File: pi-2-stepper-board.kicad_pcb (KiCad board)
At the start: 2 copper layers, 65 x 56 mm, 21 parts, among them CON1 DC12v, P1 Servo (A0), P2 Endstop1 (A1), P3 Endstop2 (A2), P4 Stepper1, P5 Stepper2, P6 COM, P7 Aux1 (D10 - 13), P8 Aux2 (I2C), SW1 SW_PUSH, SW2 SPDT, U1 Pi2_3_GPIO, U2 Arduino_Pro_Mini_3v3_8MHz, U3 STEPSTICK, U4 STEPSTICK, U5 DC2DC

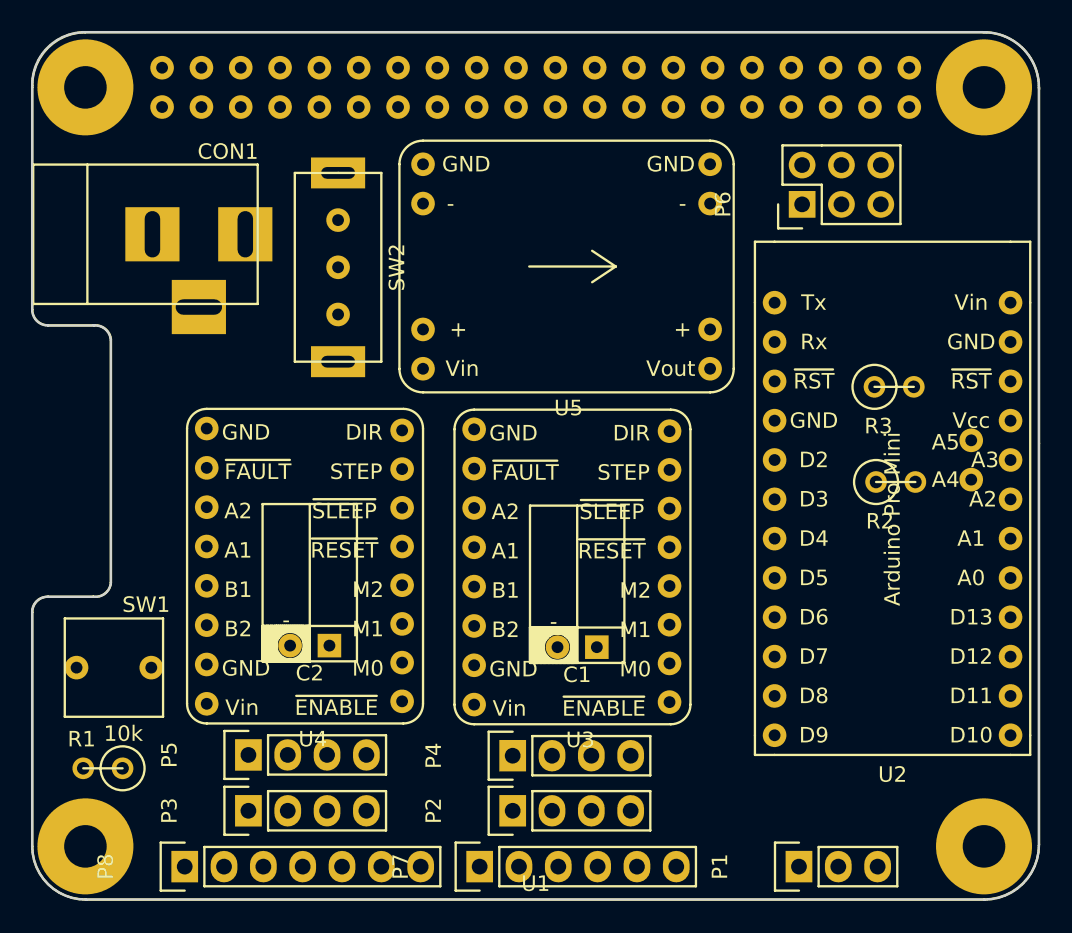
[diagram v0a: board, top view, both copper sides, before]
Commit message: Clean up repo - board 1.0a non hat spec
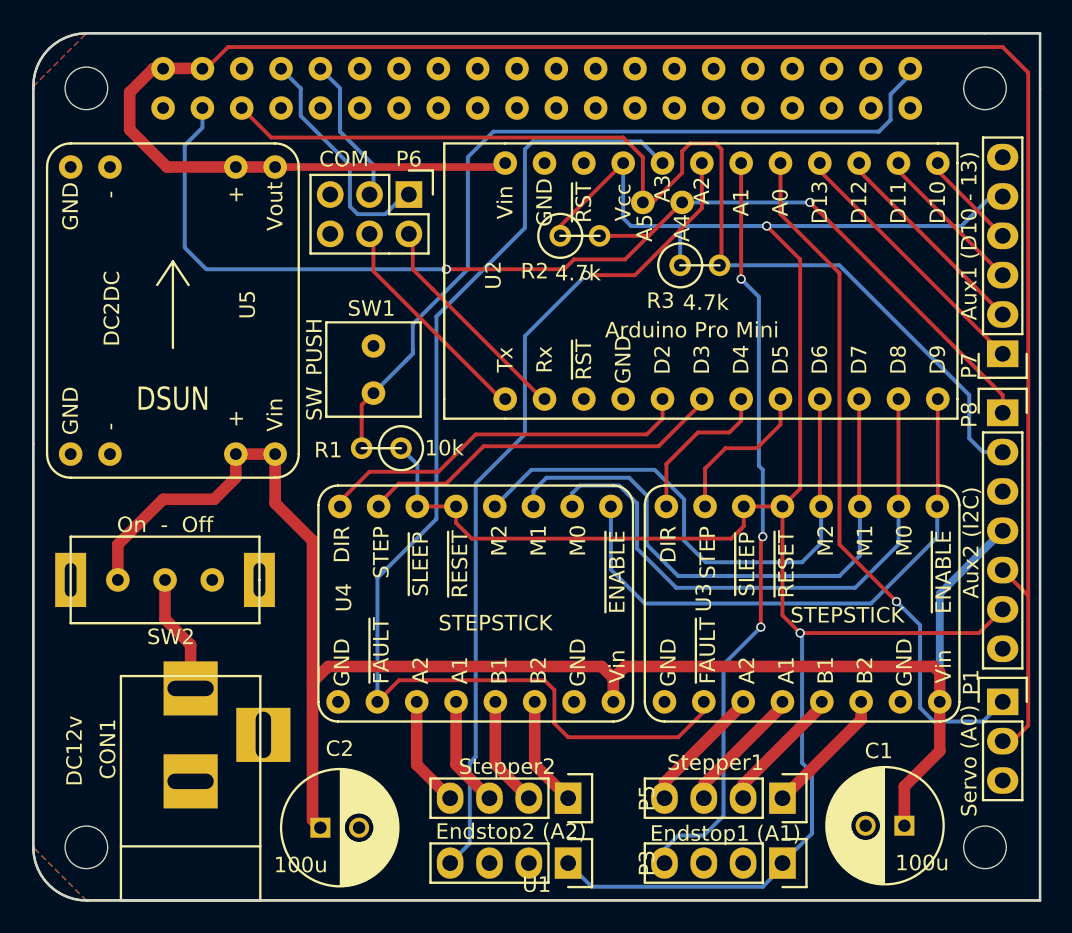
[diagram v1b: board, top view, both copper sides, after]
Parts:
- added REF**: Symbol_OSHW-Logo_SilkScreen, Symbols:Symbol_OSHW-Logo_SilkScreen, B.Cu at (86.0, 61.8)
- C1, C2: footprint custom:Cap_laying_flat_2.5mm_lead_pitch -> Capacitors_ThroughHole:C_Radial_D7.5_L11.2_P2.5
- SW2: value SPDT -> On - Off
- U1: footprint custom:Pi_2_3_Hat_spec -> custom:Pi_2_3
- moved P8 60.4 mm to (139.4, 68.6), turned to 0 degrees
- moved P7 47.3 mm to (139.4, 64.8), turned to 180 degrees
- moved CON1 35.6 mm to (87.0, 92.6), turned to 90 degrees
- moved R1 27.4 mm to (99.3, 70.9)
- moved R2 25.9 mm to (112.1, 57.1)
- moved U5 25.7 mm to (85.9, 61.8), turned to 90 degrees
- moved SW1 25.5 mm to (98.8, 65.8), turned to 90 degrees
- moved P6 25.4 mm to (101.1, 54.5), turned to 270 degrees
- moved SW2 23.1 mm to (85.3, 79.4), turned to 0 degrees
- moved C1 23.1 mm to (133.1, 95.2)
- moved P3 20.9 mm to (111.4, 97.7), turned to 270 degrees
- moved P5 20.8 mm to (111.4, 93.5), turned to 270 degrees
- moved U2 18.9 mm to (121.3, 60.1), turned to 90 degrees
- moved P2 17.7 mm to (125.2, 97.7), turned to 270 degrees
- moved P4 17.6 mm to (125.2, 93.5), turned to 270 degrees
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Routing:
- net /3v3: track 0.00 -> 142.2 mm, vias 0 -> 2
- net /VCC: track 0.00 -> 134.9 mm
- net +12V: track 0.00 -> 107.9 mm
- net /FAULT: track 0.00 -> 75.8 mm
- net /SDA: track 0.00 -> 74.2 mm, vias 0 -> 2
- net /SCL: track 0.00 -> 70.5 mm
- net /GPIO21: track 0.00 -> 54.5 mm
- net /ESTOP2: track 0.00 -> 53.8 mm, vias 0 -> 1
- net /ESTOP1: track 0.00 -> 49.4 mm, vias 0 -> 3
- net /SERVO: track 0.00 -> 45.4 mm, vias 0 -> 1
- net /M1: track 0.00 -> 37.6 mm
- net /M0: track 0.00 -> 37.1 mm
- net /ENABLE: track 0.00 -> 36.8 mm
- net /M2: track 0.00 -> 36.0 mm
- net /DIR2: track 0.00 -> 24.6 mm
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- added copper zone on B.Cu, net GND
- added copper zone on F.Cu, net GND
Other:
- outline, holes or cut-outs redrawn
- board text added: "Copyright Mark Benson 2016 License: CC-BY 4.0"
- board text added: "DSUN"
- board text added: "Designed for use with vPiP: https://github.com/brianinnes/vpip"
- board text added: "No warranty implied or given. Use at own risk!"
- board text added: "Rapsberry Pi 2/3 Arduino Pro Mini (3.3v @ 8MHz) Dual Stepper control brd"
- board text added: "https://github.com/MarkJB/pi-2-stepper-board"
